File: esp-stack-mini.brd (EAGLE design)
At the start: 53.3 x 52.1 mm, 48 parts, among them IC1 FT232RL, Q1 200mA/50V, U1 TPS737XX, U2 MCP73831

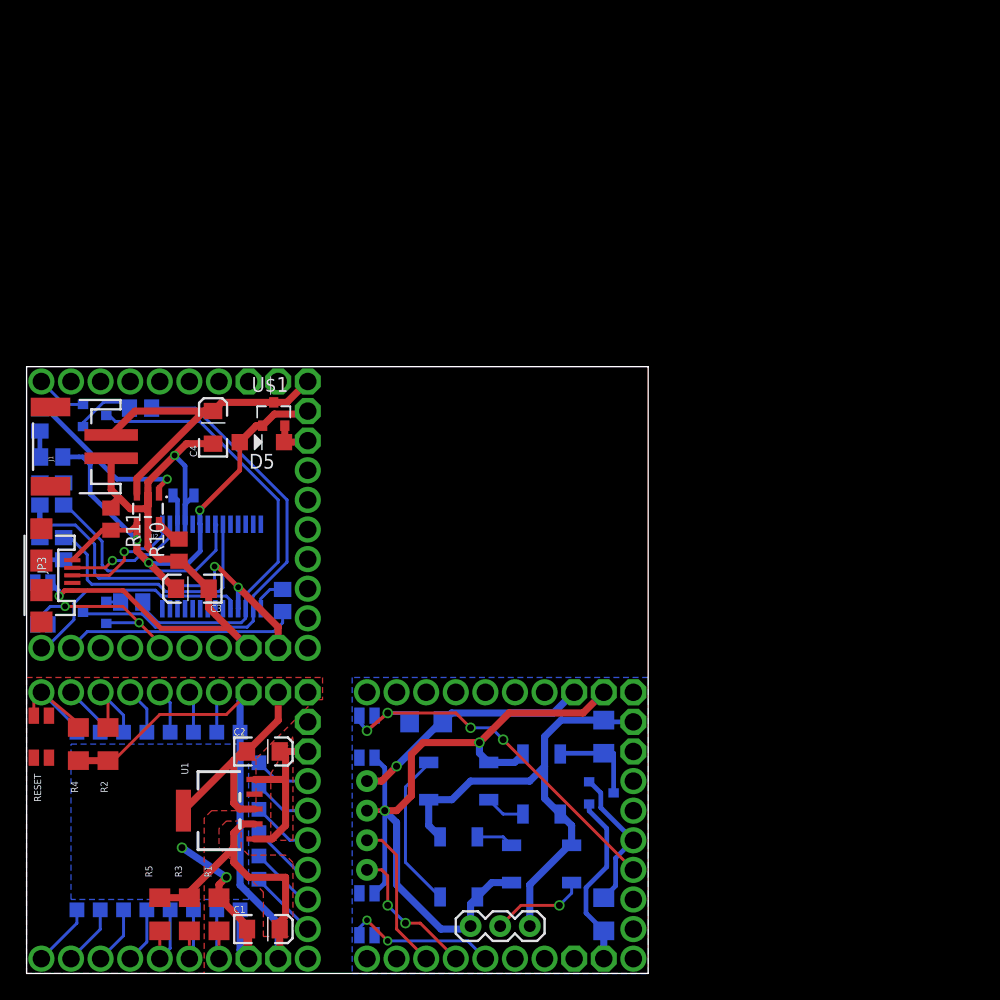
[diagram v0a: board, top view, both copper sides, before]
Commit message: First prototype
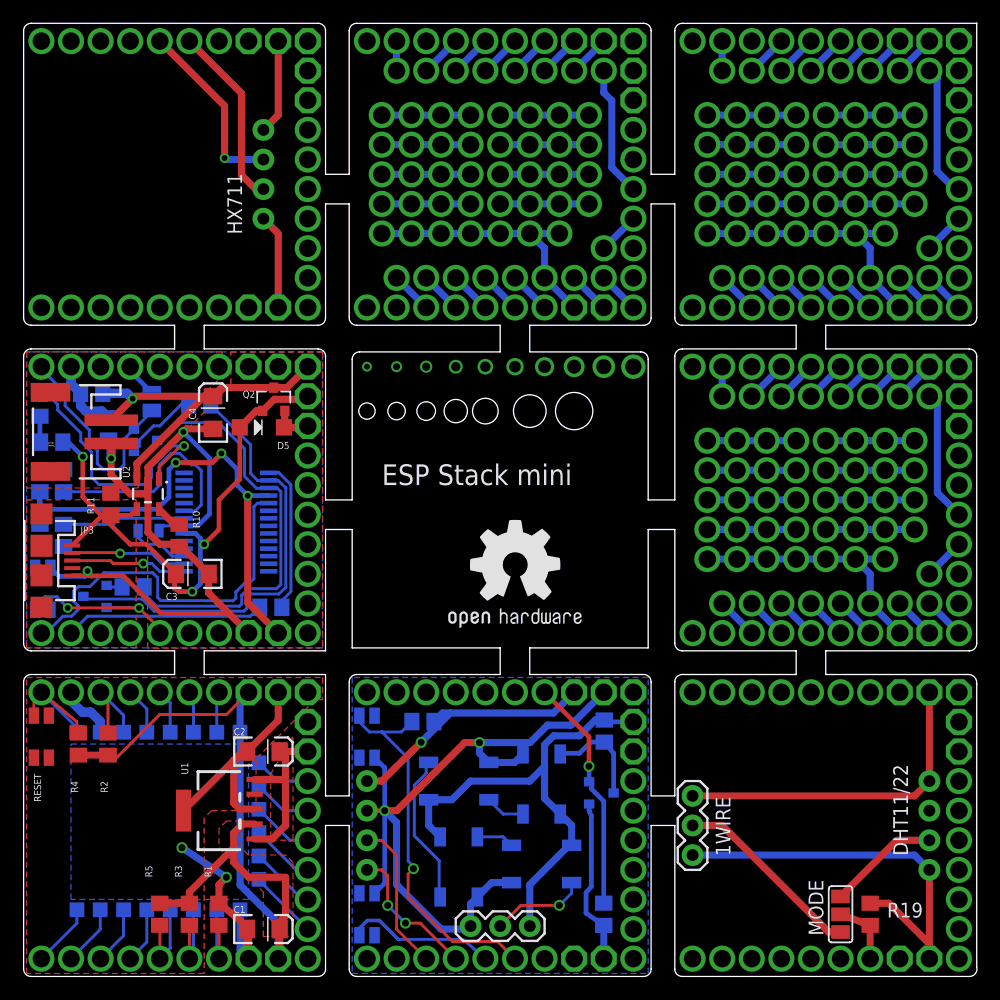
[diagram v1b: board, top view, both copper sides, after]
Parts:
- removed U$2, U$3: NPN-TRANSISTOR, ESPStack-mini:SOT23-3
- added 1WIRE: (no value), SparkFun-Connectors:1X03
- added DHT11/22, HX711: (no value), SparkFun-Connectors:1X04_NO_SILK_ALL_ROUND
- added H4, H5, H6, H7, H8: ESP-BOARD, ESPStack-mini:ESP-BOARD
- added MODE: (no value), SparkFun-Retired:SJ_2
- added Q2: AO3401, ESPStack-mini:SOT23-3
- added Q3, Q4: S8050, ESPStack-mini:SOT23-3
- added R17, R18: 470, resistor:R0805
- added R19: 4k7, resistor:R0805
- added SJ1: SLEEP, jumper:SJ
- C5: value (none) -> 100nF
- D5: value SCHOTTKY_DIODE_SMDSOD123 -> MBR120
- D7: value DIODE_SMDD0805 -> TX
- D8: value DIODE_SMDD0805 -> RX
- Q1: value 200mA/50V -> BSS138
- R1, R2, R3, R4, R5, R6, R7, R8: device resistor:R1206 -> resistor:R0805
- U$1: value P-CHANNEL-MOSFET -> (none); device ESPStack-mini:SOT23-3 -> NBitWonder:OSHW1
- moved U$1 24.7 mm to (35.6, 27.9)
- moved D7 5.84 mm to (1.14, 42.3), turned to 90 degrees
- moved R12 5.84 mm to (3.17, 42.3), turned to 270 degrees
- moved R16 5.09 mm to (14.9, 48.8)
- moved C5 4.26 mm to (10.5, 38.0)
- moved IC1 4.02 mm to (17.1, 38.7), turned to 270 degrees
- moved D8 3.56 mm to (1.14, 37.6), turned to 270 degrees
- moved R13 3.56 mm to (3.17, 37.6), turned to 90 degrees
- moved R15 1.30 mm to (9.14, 33.2)
- moved BOOT 1.27 mm to (1.40, 33.0)
- moved C4 1.27 mm to (16.0, 48.1)
- moved CHARGING 1.27 mm to (1.14, 48.8)
- moved JP3 1.27 mm to (1.27, 35.4)
- moved R11 1.27 mm to (7.24, 40.3)
- moved R9 1.27 mm to (2.16, 45.6)
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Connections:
- new net 1WIRE: 1WIRE.2, MODE.3
- new net DHT: DHT11/22.2, MODE.1
- net 3V3: now also 1WIRE.1, DHT11/22.1, H4.3V3@1, H4.3V3@2, H5.3V3@1, H5.3V3@2, H6.3V3@1, H6.3V3@2, H7.3V3@1, H7.3V3@2, H8.3V3@1, H8.3V3@2, HX711.1, R19.2
- net ADC: now also H3.ADC, H6.ADC, H7.ADC, H8.ADC, R17.1, R18.2
- net D0: now also H6.D0, H7.D0, H8.D0, Q3.2; no longer U$2.2
- net D10: now also H6.D10, H7.D10, H8.D10; no longer B1.2, H2.D10, R6.1
- net D12: now also H4.D12, H6.D12, H7.D12, H8.D12, HX711.2
- net D13: now also H2.D13, H6.D13, H7.D13, H8.D13, Q1.2, R7.1
- net D14: now also H4.D14, H6.D14, H7.D14, H8.D14, HX711.3
- net D15: now also H5.D15, H6.D15, H7.D15, H8.D15, MODE.2, R19.1
- net D16: now also H3.D16, H6.D16, H7.D16, H8.D16, SJ1.2
- net D2: now also B1.2, H2.D2, H6.D2, H7.D2, H8.D2, R6.1
- net D4: now also H6.D4, H7.D4, H8.D4
- net D5: now also H6.D5, H7.D5, H8.D5
- net D9: now also H6.D9, H7.D9, H8.D9; no longer H2.D9, Q1.2, R7.1
- net GND: now also 1WIRE.3, DHT11/22.4, H4.GND@1, H4.GND@2, H5.GND@1, H5.GND@2, H6.GND@1, H6.GND@2, H7.GND@1, H7.GND@2, H8.GND@1, H8.GND@2, HX711.4, R18.1
- net N$15: now also Q4.3; no longer U$3.3
- net N$16: now also Q3.3; no longer U$2.3
- net N$8: now also Q4.1; no longer U$3.1
- net N$9: now also Q3.1; no longer U$2.1
- net RST: now also Q4.2, SJ1.1; no longer U$3.2
- net S1: now also H6.S1, H7.S1, H8.S1
- net V+: now also H4.V+, H5.V+, H6.V+, H7.V+, H8.V+, Q2.2; no longer U$1.2
- net VBATT: now also H4.VBATT, H5.VBATT, H6.VBATT, H7.VBATT, H8.VBATT, Q2.3, R17.2; no longer U$1.3
- net VBUS: now also H4.VBUS, H5.VBUS, H6.VBUS, H7.VBUS, H8.VBUS, Q2.1; no longer U$1.1
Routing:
- net GND: track 166.7 -> 289.1 mm, vias 6 -> 34
- net 3V3: track 138.7 -> 211.7 mm, vias 3 -> 10
- net D2: track 6.73 -> 50.6 mm, vias 0 -> 4
- net D13: track 3.51 -> 34.5 mm, vias 0 -> 4
- net D14: track 3.80 -> 30.3 mm, vias 0 -> 4
- net D12: track 3.57 -> 30.1 mm, vias 0 -> 3
- net D10: track 38.3 -> 16.3 mm, vias 4 -> 3
- net D9: track 17.9 -> 39.1 mm, vias 0 -> 3
- net D15: track 6.66 -> 23.5 mm, vias 0 -> 3
- net 1WIRE: track 0.00 -> 16.5 mm
- net RST: track 15.8 -> 30.5 mm
- net ADC: track 4.47 -> 19.0 mm, vias 0 -> 3
- net D16: track 4.02 -> 17.8 mm, vias 0 -> 3
- net TX: track 25.7 -> 38.0 mm
- net N$13: track 2.25 -> 13.2 mm
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- added copper zone on layer 1, net VBATT
- added copper zone on layer 1, net VBUS
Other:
- board size 53.3 x 52.1 mm -> 81.8 x 81.8 mm
- board text added: "ESP Stack mini"
